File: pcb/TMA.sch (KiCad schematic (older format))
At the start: 22 parts, among them J1 Conn_01x02, J2 Conn_01x06, SW1 SW_SPDT, U1 BMP280, U2 BMI160, U3 ATtiny1614-SS, U4 MIC5504-3.3YM5

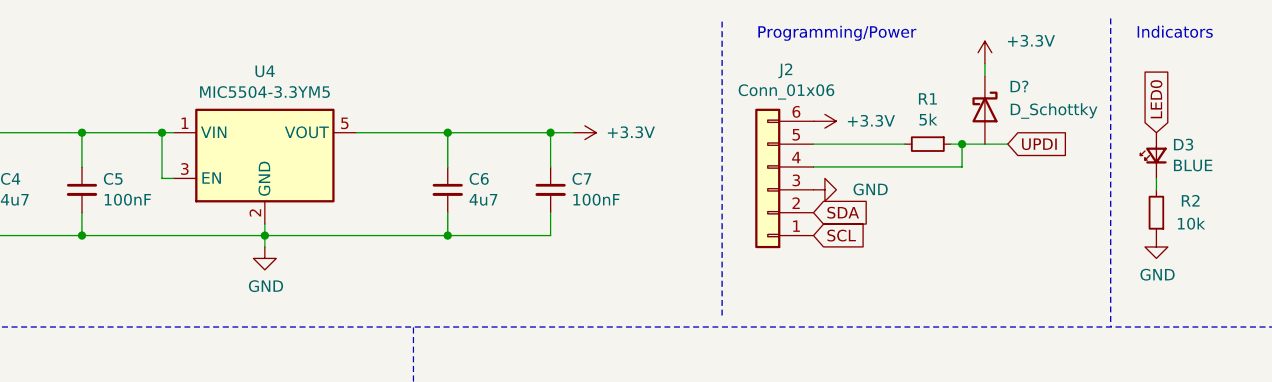
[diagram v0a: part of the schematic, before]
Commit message: Pick components.
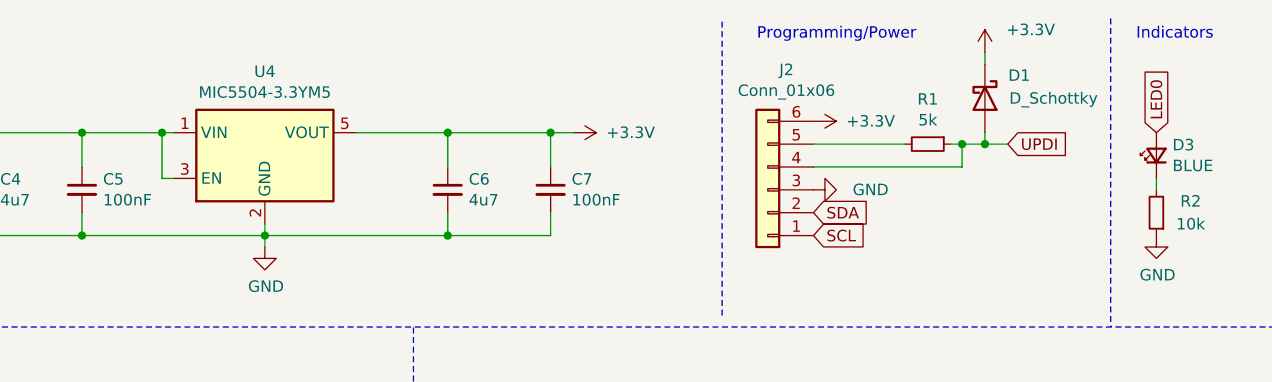
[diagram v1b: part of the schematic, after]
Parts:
- C1, C2, C3, C4, C5, C6, C7: footprint (none) -> Capacitor_SMD:C_0402_1005Metric
- D1: renamed from D?; footprint (none) -> Diode_SMD:D_0402_1005Metric
- D3, D4: footprint (none) -> LED_SMD:LED_0402_1005Metric
- J1: footprint (none) -> Connector_JST:JST_PH_B2B-PH-K_1x02_P2.00mm_Vertical
- J2: footprint (none) -> Connector_JST:JST_PH_B6B-PH-K_1x06_P2.00mm_Vertical
- R1, R2, R3, R4, R5: footprint (none) -> Resistor_SMD:R_0402_1005Metric
- SW1: footprint (none) -> Button_Switch_SMD:SW_SPDT_PCM12
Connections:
- net UPDI: now also D1.2 (A)
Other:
- moved on the sheet: D1
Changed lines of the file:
@@
 F 0 "C1" H 2092 3346 50  0000 L CNN
 F 1 "100nF" H 2092 3255 50  0000 L CNN
-F 2 "" H 2000 3300 50  0001 C CNN
+F 2 "Capacitor_SMD:C_0402_1005Metric" H 2000 3300 50  0001 C CNN
 F 3 "~" H 2000 3300 50  0001 C CNN
 	1    2000 3300
@@
 F 0 "C2" H 2242 1096 50  0000 L CNN
 F 1 "100nF" H 2242 1005 50  0000 L CNN
-F 2 "" H 2150 1050 50  0001 C CNN
+F 2 "Capacitor_SMD:C_0402_1005Metric" H 2150 1050 50  0001 C CNN
 F 3 "~" H 2150 1050 50  0001 C CNN
 	1    2150 1050
@@
 F 0 "J1" H 2818 775 50  0000 C CNN
 F 1 "Conn_01x02" H 2818 866 50  0000 C CNN
-F 2 "" H 2900 1100 50  0001 C CNN
+F 2 "Connector_JST:JST_PH_B2B-PH-K_1x02_P2.00mm_Vertical" H 2900 1100 50  0001 C CNN
 F 3 "~" H 2900 1100 50  0001 C CNN
 	1    2900 1100
@@
 F 0 "C3" H 2942 2796 50  0000 L CNN
 F 1 "100nF" H 2942 2705 50  0000 L CNN
-F 2 "" H 2850 2750 50  0001 C CNN
+F 2 "Capacitor_SMD:C_0402_1005Metric" H 2850 2750 50  0001 C CNN
 F 3 "~" H 2850 2750 50  0001 C CNN
 	1    2850 2750
@@
 F 0 "C4" H 3592 1296 50  0000 L CNN
 F 1 "4u7" H 3592 1205 50  0000 L CNN
-F 2 "" H 3500 1250 50  0001 C CNN
+F 2 "Capacitor_SMD:C_0402_1005Metric" H 3500 1250 50  0001 C CNN
 F 3 "~" H 3500 1250 50  0001 C CNN
 	1    3500 1250
@@
 F 0 "C5" H 4042 1296 50  0000 L CNN
 F 1 "100nF" H 4042 1205 50  0000 L CNN
-F 2 "" H 3950 1250 50  0001 C CNN
+F 2 "Capacitor_SMD:C_0402_1005Metric" H 3950 1250 50  0001 C CNN
 F 3 "~" H 3950 1250 50  0001 C CNN
 	1    3950 1250
@@
 $EndComp
 Connection ~ 3950 1000
-Wire Wire Line
-	3950 1000 4300 1000
 $Comp
 L power:GND #PWR09
@@
 F 0 "C6" H 5642 1296 50  0000 L CNN
 F 1 "4u7" H 5642 1205 50  0000 L CNN
-F 2 "" H 5550 1250 50  0001 C CNN
+F 2 "Capacitor_SMD:C_0402_1005Metric" H 5550 1250 50  0001 C CNN
 F 3 "~" H 5550 1250 50  0001 C CNN
 	1    5550 1250
@@
 F 0 "C7" H 6092 1296 50  0000 L CNN
 F 1 "100nF" H 6092 1205 50  0000 L CNN
-F 2 "" H 6000 1250 50  0001 C CNN
+F 2 "Capacitor_SMD:C_0402_1005Metric" H 6000 1250 50  0001 C CNN
 F 3 "~" H 6000 1250 50  0001 C CNN
 	1    6000 1250
@@
 Wire Wire Line
 	4750 1500 4750 1450
-Wire Wire Line
-	4300 1000 4300 1200
-Wire Wire Line
-	4300 1200 4350 1200
-Connection ~ 4300 1000
-Wire Wire Line
-	4300 1000 4350 1000
 $Comp
 L power:+3.3V #PWR010
@@
 F 0 "R1" V 7454 1050 50  0000 C CNN
 F 1 "5k" V 7545 1050 50  0000 C CNN
-F 2 "" H 7650 1050 50  0001 C CNN
+F 2 "Resistor_SMD:R_0402_1005Metric" H 7650 1050 50  0001 C CNN
 F 3 "~" H 7650 1050 50  0001 C CNN
 	1    7650 1050
@@
 F 0 "J2" H 6868 725 50  0000 C CNN
 F 1 "Conn_01x06" H 6868 816 50  0000 C CNN
-F 2 "" H 6950 1250 50  0001 C CNN
+F 2 "Connector_JST:JST_PH_B6B-PH-K_1x06_P2.00mm_Vertical" H 6950 1250 50  0001 C CNN
 F 3 "~" H 6950 1250 50  0001 C CNN
 	1    6950 1250
@@
 F 0 "D3" V 8696 1030 50  0000 R CNN
 F 1 "BLUE" V 8605 1030 50  0000 R CNN
-F 2 "" V 8650 1100 50  0001 C CNN
+F 2 "LED_SMD:LED_0402_1005Metric" V 8650 1100 50  0001 C CNN
 F 3 "~" V 8650 1100 50  0001 C CNN
 	1    8650 1100
@@
 F 0 "D4" V 9496 1030 50  0000 R CNN
 F 1 "RED" V 9405 1030 50  0000 R CNN
-F 2 "" V 9450 1100 50  0001 C CNN
+F 2 "LED_SMD:LED_0402_1005Metric" V 9450 1100 50  0001 C CNN
 F 3 "~" V 9450 1100 50  0001 C CNN
 	1    9450 1100
@@
 F 0 "R2" H 8500 1300 50  0000 C CNN
 F 1 "10k" H 8500 1400 50  0000 C CNN
-F 2 "" H 8650 1350 50  0001 C CNN
+F 2 "Resistor_SMD:R_0402_1005Metric" H 8650 1350 50  0001 C CNN
 F 3 "~" H 8650 1350 50  0001 C CNN
 	1    8650 1350
@@
 F 0 "R3" H 9300 1300 50  0000 C CNN
 F 1 "10k" H 9300 1400 50  0000 C CNN
-F 2 "" H 9450 1350 50  0001 C CNN
+F 2 "Resistor_SMD:R_0402_1005Metric" H 9450 1350 50  0001 C CNN
 F 3 "~" H 9450 1350 50  0001 C CNN
 	1    9450 1350
@@
 F 0 "R4" V 10400 900 50  0000 C CNN
 F 1 "10k" V 10400 1050 50  0000 C CNN
-F 2 "" H 10500 1000 50  0001 C CNN
+F 2 "Resistor_SMD:R_0402_1005Metric" H 10500 1000 50  0001 C CNN
 F 3 "~" H 10500 1000 50  0001 C CNN
 	1    10500 1000
@@
 F 0 "R5" V 10400 700 50  0000 C CNN
 F 1 "10k" V 10400 850 50  0000 C CNN
-F 2 "" H 10500 800 50  0001 C CNN
+F 2 "Resistor_SMD:R_0402_1005Metric" H 10500 800 50  0001 C CNN
 F 3 "~" H 10500 800 50  0001 C CNN
 	1    10500 800
@@
 F 0 "SW1" H 10350 1350 50  0000 C CNN
 F 1 "SW_SPDT" H 10350 1450 50  0000 C CNN
-F 2 "" H 10550 1600 50  0001 C CNN
+F 2 "Button_Switch_SMD:SW_SPDT_PCM12" H 10550 1600 50  0001 C CNN
 F 3 "~" H 10550 1600 50  0001 C CNN
 	1    10550 1600
@@
 MODE
 Wire Wire Line
-	7800 1050 8000 1050
+	7800 1050 7900 1050
 Wire Wire Line
 	10600 800  10700 800
@@
 Connection ~ 10700 800
 $Comp
-L power:+3.3V #PWR?
+L power:+3.3V #PWR0107
 U 1 1 607905AF
-P 7900 700
-F 0 "#PWR?" H 7900 550 50  0001 C CNN
-F 1 "+3.3V" H 8100 800 50  0000 C CNN
-F 2 "" H 7900 700 50  0001 C CNN
-F 3 "" H 7900 700 50  0001 C CNN
-	1    7900 700
-	1    0    0    -1
-$EndComp
-$Comp
-L Device:D_Schottky D?
+P 7900 650
+F 0 "#PWR0107" H 7900 500 50  0001 C CNN
+F 1 "+3.3V" H 8100 750 50  0000 C CNN
+F 2 "" H 7900 650 50  0001 C CNN
+F 3 "" H 7900 650 50  0001 C CNN
+	1    7900 650
+	1    0    0    -1
+$EndComp
+$Comp
+L Device:D_Schottky D1
 U 1 1 607905B5
-P 7900 900
-F 0 "D?" V 7800 1050 50  0000 C CNN
-F 1 "D_Schottky" V 7900 1200 50  0000 C CNN
-F 2 "" H 7900 900 50  0001 C CNN
-F 3 "~" H 7900 900 50  0001 C CNN
-	1    7900 900
-	0    1    1    0
-$EndComp
-Wire Wire Line
-	7900 750  7900 700
+P 7900 850
+F 0 "D1" V 7800 1000 50  0000 C CNN
+F 1 "D_Schottky" V 7900 1150 50  0000 C CNN
+F 2 "Diode_SMD:D_0402_1005Metric" H 7900 850 50  0001 C CNN
+F 3 "~" H 7900 850 50  0001 C CNN
+	1    7900 850
+	0    1    1    0
+$EndComp
+Wire Wire Line
+	7900 700  7900 650
 Wire Notes Line
 	5400 4650 5400 1850
@@
 Wire Wire Line
 	6000 1000 6100 1000
+Wire Wire Line
+	7900 1050 7900 1000
+Connection ~ 7900 1050
+Wire Wire Line
+	7900 1050 8000 1050
+Wire Wire Line
+	3950 1000 4300 1000
+Wire Wire Line
+	4350 1200 4300 1200
+Wire Wire Line
+	4300 1200 4300 1000
+Connection ~ 4300 1000
+Wire Wire Line
+	4300 1000 4350 1000
 $EndSCHEMATC
